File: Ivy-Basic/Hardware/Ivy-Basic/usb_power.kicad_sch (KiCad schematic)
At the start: 6 parts, among them J1 USB_C_Receptacle_USB2.0_16P

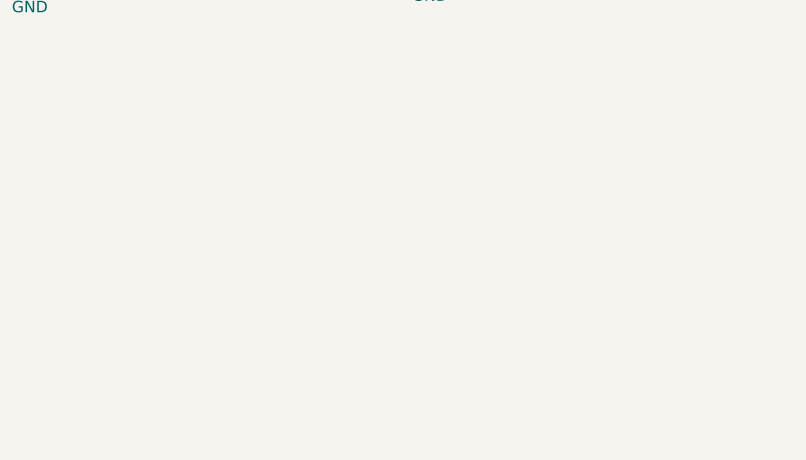
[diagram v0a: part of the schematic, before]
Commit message: ti switcher
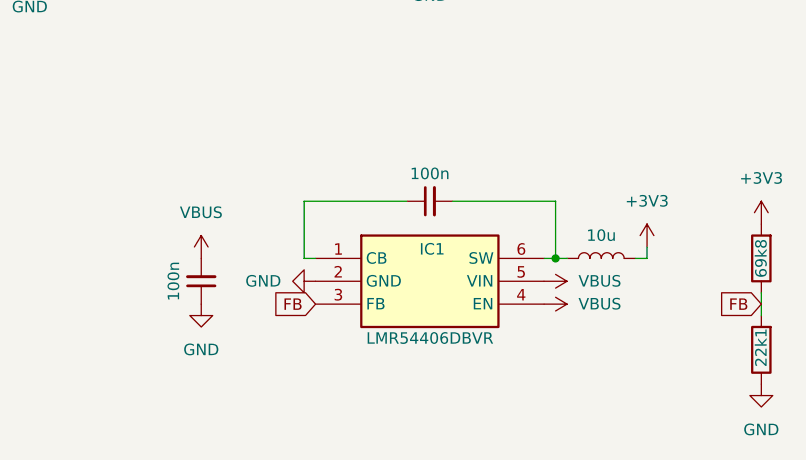
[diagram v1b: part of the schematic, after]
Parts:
- added C10, C11: 100n, Capacitor_SMD:C_0402_1005Metric, symbol Device:C_Small
- added IC1: LMR54406DBVR, SOT95P280X145-6N, symbol LMR54406DBVR:LMR54406DBVR
- added L1: 10u, symbol Device:L
- added R5: 69k8, symbol Device:R
- added R6: 22k1, symbol Device:R
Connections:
- net +3V3: now also L1.2, R5.2
- net GND: now also C11.1, IC1.2 (GND), R6.1
- net VBUS: now also C11.2, IC1.4 (EN), IC1.5 (VIN)
- new net: C10.1, IC1.1 (CB)
- new net: C10.2, IC1.6 (SW), L1.1
- new net FB: IC1.3 (FB), R5.1, R6.2
